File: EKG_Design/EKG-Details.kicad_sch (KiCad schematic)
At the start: 43 parts, among them J1 Conn_01x02_Pin, J2 Conn_01x02_Pin, J3 Conn_01x02_Pin, J4 Conn_01x03_Pin, J5 Conn_01x02_Pin, U1 OPA2156xDGK, U2 OPA2156xDGK, U3 OPA2156xDGK, U4 OPA2156xDGK, U5 OPA2156xDGK

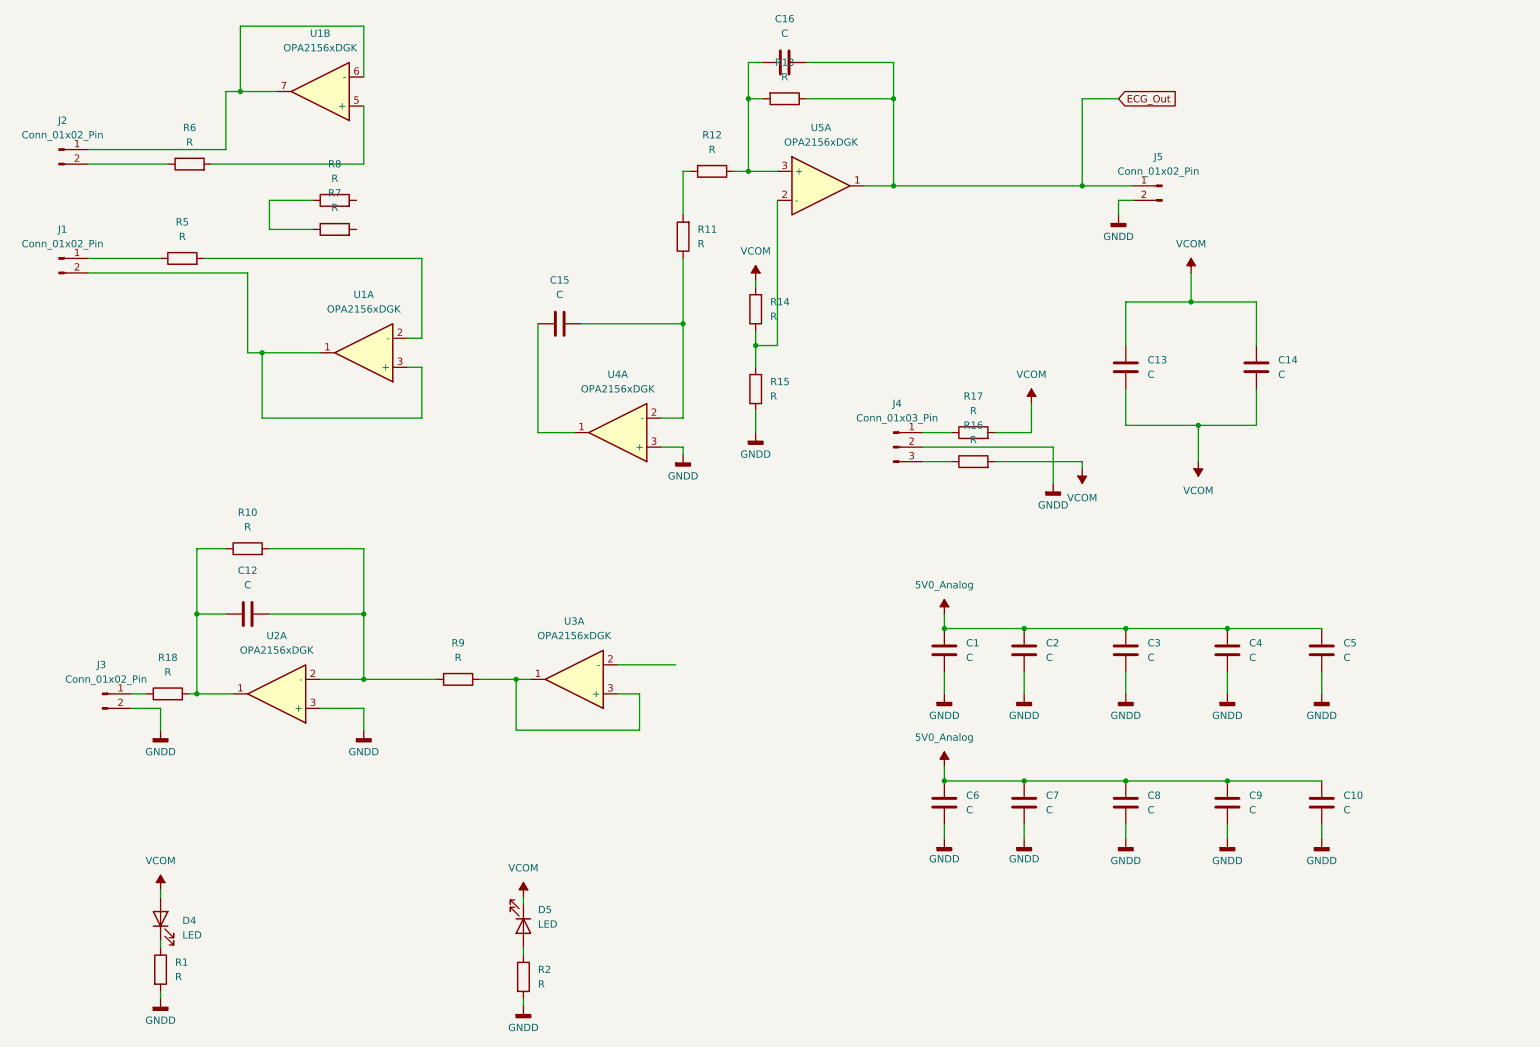
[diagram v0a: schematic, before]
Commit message: Finished EKG Schematic
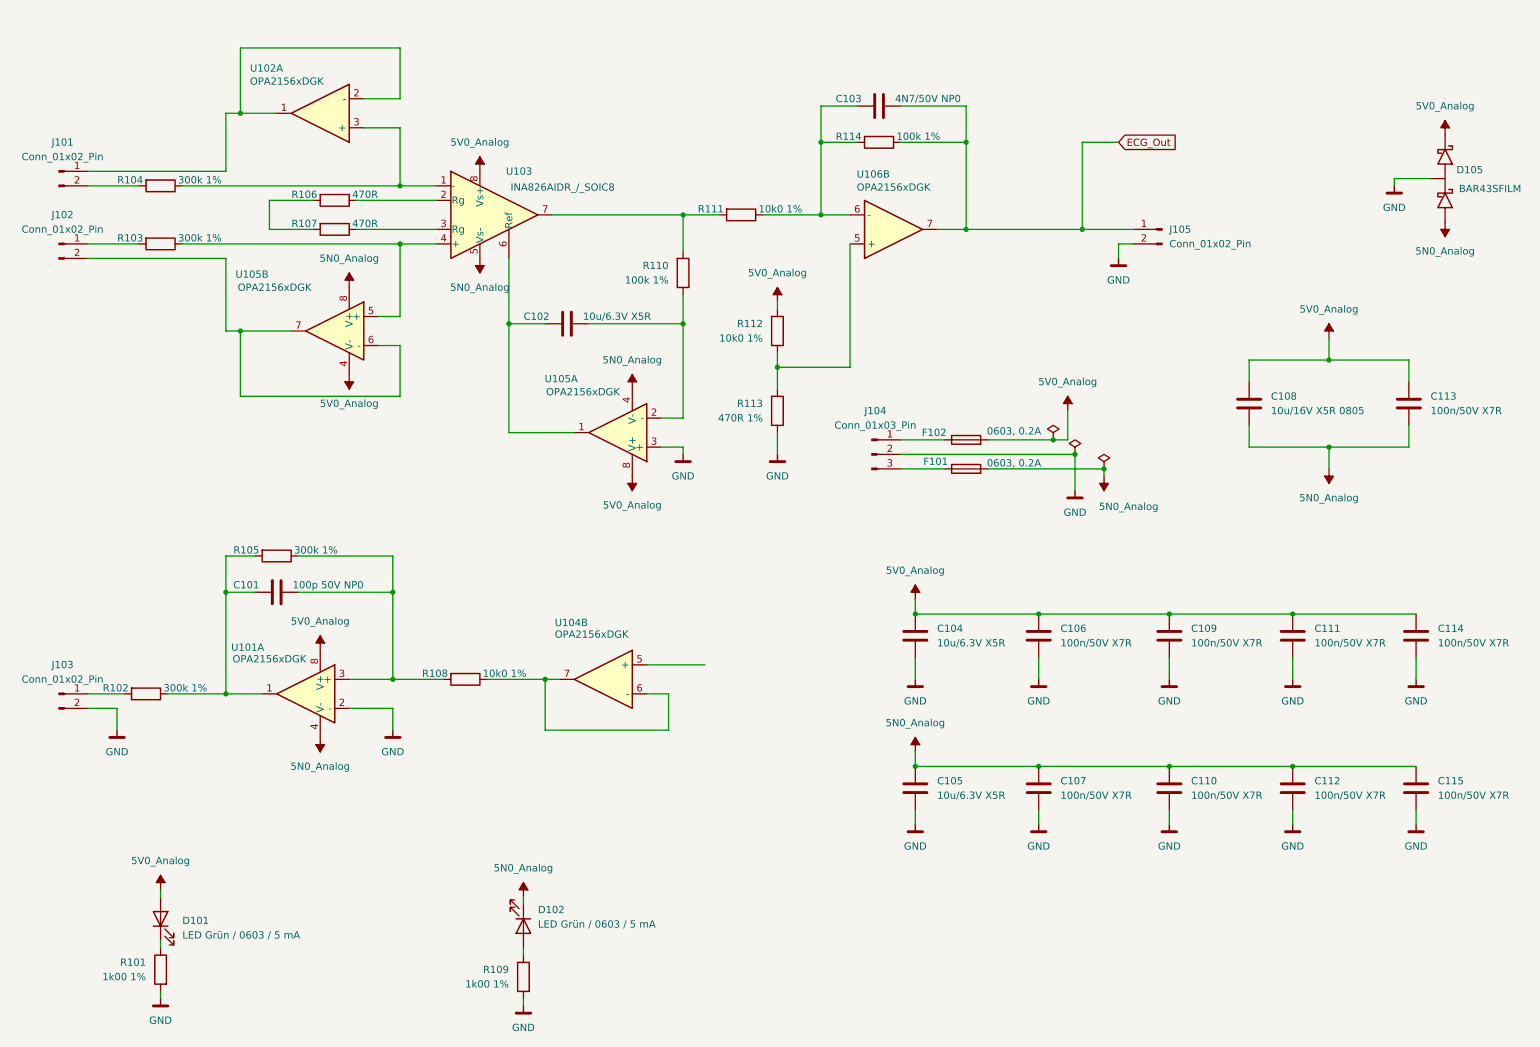
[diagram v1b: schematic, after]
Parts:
- removed R16, R17: R, symbol Device:R
- removed unit 1 of U1
- added D105: BAR43SFILM, Package_TO_SOT_SMD:SOT-23, symbol CustomSymbols:BAR43SFILM
- added F101, F102: 0603, 0.2A, symbol Device:Fuse
- added unit 1 of U101
- added unit 3 of U102
- added U103: INA826AIDR_/_SOIC8, Package_SO:SOIC-8_3.9x4.9mm_P1.27mm, symbol Amplifier_Instrumentation:INA821xD
- added unit 3 of U105
- added unit 2 of U105
- C101: renamed from C12; value C -> 100p 50V NP0; symbol Device:C -> Custom_Device:C
- C102: renamed from C15; value C -> 10u/6.3V X5R; symbol Device:C -> Custom_Device:C
- C103: renamed from C16; value C -> 4N7/50V NP0; symbol Device:C -> Custom_Device:C
- C104: renamed from C1; value C -> 10u/6.3V X5R
- C105: renamed from C6; value C -> 10u/6.3V X5R
- C106: renamed from C2; value C -> 100n/50V X7R
- C107: renamed from C7; value C -> 100n/50V X7R
- C108: renamed from C13; value C -> 10u/16V X5R 0805
- C109: renamed from C3; value C -> 100n/50V X7R
- C110: renamed from C8; value C -> 100n/50V X7R
- C111: renamed from C4; value C -> 100n/50V X7R
- C112: renamed from C9; value C -> 100n/50V X7R
- C113: renamed from C14; value C -> 100n/50V X7R
- C114: renamed from C5; value C -> 100n/50V X7R
- C115: renamed from C10; value C -> 100n/50V X7R
- D101: renamed from D4; value LED -> LED Grün / 0603 / 5 mA
- D102: renamed from D5; value LED -> LED Grün / 0603 / 5 mA
- R101: renamed from R1; value R -> 1k00 1%
- R102: renamed from R18; value R -> 300k 1%; symbol Device:R -> Custom_Device:R
- R103: renamed from R5; value R -> 300k 1%; symbol Device:R -> Custom_Device:R
- R104: renamed from R6; value R -> 300k 1%; symbol Device:R -> Custom_Device:R
- R105: renamed from R10; value R -> 300k 1%; symbol Device:R -> Custom_Device:R
- R106: renamed from R8; value R -> 470R; symbol Device:R -> Custom_Device:R
- R107: renamed from R7; value R -> 470R; symbol Device:R -> Custom_Device:R
- R108: renamed from R9; value R -> 10k0 1%; symbol Device:R -> Custom_Device:R
- R109: renamed from R2; value R -> 1k00 1%
- R110: renamed from R11; value R -> 100k 1%
- R111: renamed from R12; value R -> 10k0 1%; symbol Device:R -> Custom_Device:R
- R112: renamed from R14; value R -> 10k0 1%
- R113: renamed from R15; value R -> 470R 1%
- R114: renamed from R13; value R -> 100k 1%; symbol Device:R -> Custom_Device:R
- renumbered J2 to J101, J1 to J102, J3 to J103, J4 to J104, J5 to J105, U2 to U101, U1 to U102, U3 to U104, U4 to U105, U5 to U106
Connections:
- net 5V0_Analog: now also C108.1, C113.1, D101.2 (A), R112.2, U101.8 (V+), D105.3 (K), F102.2, U102.4 (V-), U103.8 (Vs+), U105.8 (V+); no longer C105.1, C107.1, C110.1, C112.1, C115.1
- net ECG_Out: now also C103.1, U106.7; no longer C103.2, U106.1
- net at R111.1, R114.2: now also C103.2, U106.6 (-); no longer C103.1, U106.3 (+)
- net at R110.2, R111.2: now also U103.7
- net at C101.1, R105.1: now also R108.2, U101.3 (+); no longer R102.2, U101.1
- net at C101.2, R105.2: now also R102.1, U101.1; no longer R108.1, U101.2 (-)
- net at R104.2: now also J101.2 (Pin_2); no longer U102.5 (+)
- net at J103.1 (Pin_1): now also R102.2; no longer R102.1
- net at C102.1: now also R110.1, U105.2 (-); no longer U105.1
- net at R112.1, R113.2: now also U106.5 (+); no longer U106.2 (-)
- net at R103.1: now also U103.4 (+), U105.5 (+); no longer J102.1 (Pin_1)
- net at R103.2: now also J102.1 (Pin_1)
- net at R106.1: now also U103.2 (Rg); no longer R107.1
- net at R106.2: now also R107.2
- net at J102.2 (Pin_2): now also U105.6 (-), U105.7
- net at J104.1 (Pin_1): now also F102.1
- net at R104.1: now also U102.3 (+), U103.1 (-); no longer J101.2 (Pin_2)
- net at J104.3 (Pin_3): now also F101.1
- net GNDD renamed GND
- net GND: now also D105.1 (A), U101.2 (-); no longer U101.3 (+)
- removed net VCOM: C108.1, C108.2, C113.1, C113.2, D101.2 (A), D102.1 (K), R112.2
- new net: J101.1 (Pin_1), U102.1, U102.2 (-)
- new net: C102.2, U103.6 (Ref), U105.1
- new net: R108.1, U104.6 (-), U104.7
- new net: R107.1, U103.3 (Rg)
- new net 5N0_Analog: C105.1, C107.1, C108.2, C110.1, C112.1, C113.2, C115.1, D102.1 (K), D105.1 (A), F101.2, U101.4 (V-), U102.8 (V+), U103.5 (Vs-), U105.4 (V-)
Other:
- moved on the sheet: C101, C102, C103, C104, C105, C106, C107, C108, C109, C110, C111, C112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
